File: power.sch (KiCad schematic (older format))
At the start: 32 parts, among them SW1 SW_DPST_x2, U1 SPX3819-1.8, U2 IMP811REUS-T, U3 SP6205EM5-L-3-3_TR, U4 MP1469GJ

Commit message: finished scimatic for now, and started populating PCB. *chugs rrum*
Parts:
- C1, C10, C11, C12, C13, C14, C15, C2, C3, C4, C5, C6, C7, C8, C9: footprint (none) -> Capacitor_SMD:C_0402_1005Metric
- L1, L2: footprint (none) -> Inductor_SMD:L_0402_1005Metric
- R1, R2, R3, R4, R5, R6, R7, R8, R9: footprint (none) -> Resistor_SMD:R_0402_1005Metric
- SW1, U2: footprint (none) -> Package_TO_SOT_SMD:SOT-543
- U1: footprint (none) -> Package_TO_SOT_SMD:SOT-23-5
- U4: footprint (none) -> Package_TO_SOT_SMD:SOT-223-6
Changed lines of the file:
@@
 $Descr A4 11693 8268
 encoding utf-8
-Sheet 2 4
+Sheet 2 5
 Title ""
 Date ""
@@
 F 0 "R3" V 3743 2350 50  0000 C CNN
 F 1 "100k" V 3834 2350 50  0000 C CNN
-F 2 "" V 3880 2350 50  0001 C CNN
+F 2 "Resistor_SMD:R_0402_1005Metric" V 3880 2350 50  0001 C CNN
 F 3 "~" H 3950 2350 50  0001 C CNN
 	1    3950 2350
@@
 F 0 "C10" H 5915 1946 50  0000 L CNN
 F 1 "10nF" H 5915 1855 50  0000 L CNN
-F 2 "" H 5838 1750 50  0001 C CNN
+F 2 "Capacitor_SMD:C_0402_1005Metric" H 5838 1750 50  0001 C CNN
 F 3 "~" H 5800 1900 50  0001 C CNN
 	1    5800 1900
@@
 F 0 "C9" H 5515 1946 50  0000 L CNN
 F 1 "10nF" H 5515 1855 50  0000 L CNN
-F 2 "" H 5438 1750 50  0001 C CNN
+F 2 "Capacitor_SMD:C_0402_1005Metric" H 5438 1750 50  0001 C CNN
 F 3 "~" H 5400 1900 50  0001 C CNN
 	1    5400 1900
@@
 F 0 "C2" H 2565 1946 50  0000 L CNN
 F 1 "C" H 2565 1855 50  0000 L CNN
-F 2 "" H 2488 1750 50  0001 C CNN
+F 2 "Capacitor_SMD:C_0402_1005Metric" H 2488 1750 50  0001 C CNN
 F 3 "~" H 2450 1900 50  0001 C CNN
 	1    2450 1900
@@
 F 0 "R6" V 7993 1550 50  0000 C CNN
 F 1 "33R" V 8084 1550 50  0000 C CNN
-F 2 "" V 8130 1550 50  0001 C CNN
+F 2 "Resistor_SMD:R_0402_1005Metric" V 8130 1550 50  0001 C CNN
 F 3 "~" H 8200 1550 50  0001 C CNN
 	1    8200 1550
@@
 F 0 "R9" H 8570 1796 50  0000 L CNN
 F 1 "1K" H 8570 1705 50  0000 L CNN
-F 2 "" V 8430 1750 50  0001 C CNN
+F 2 "Resistor_SMD:R_0402_1005Metric" V 8430 1750 50  0001 C CNN
 F 3 "~" H 8500 1750 50  0001 C CNN
 	1    8500 1750
@@
 F 0 "C13" H 8965 1796 50  0000 L CNN
 F 1 "10uF" H 8965 1705 50  0000 L CNN
-F 2 "" H 8888 1600 50  0001 C CNN
+F 2 "Capacitor_SMD:C_0402_1005Metric" H 8888 1600 50  0001 C CNN
 F 3 "~" H 8850 1750 50  0001 C CNN
 	1    8850 1750
@@
 F 0 "C1" H 1065 3846 50  0000 L CNN
 F 1 "100nF" H 1065 3755 50  0000 L CNN
-F 2 "" H 988 3650 50  0001 C CNN
+F 2 "Capacitor_SMD:C_0402_1005Metric" H 988 3650 50  0001 C CNN
 F 3 "~" H 950 3800 50  0001 C CNN
 	1    950  3800
@@
 F 0 "R1" V 1343 3800 50  0000 C CNN
 F 1 "100K" V 1434 3800 50  0000 C CNN
-F 2 "" V 1480 3800 50  0001 C CNN
+F 2 "Resistor_SMD:R_0402_1005Metric" V 1480 3800 50  0001 C CNN
 F 3 "~" H 1550 3800 50  0001 C CNN
 	1    1550 3800
@@
 F 0 "C3" H 3115 3996 50  0000 L CNN
 F 1 "10nF" H 3115 3905 50  0000 L CNN
-F 2 "" H 3038 3800 50  0001 C CNN
+F 2 "Capacitor_SMD:C_0402_1005Metric" H 3038 3800 50  0001 C CNN
 F 3 "~" H 3000 3950 50  0001 C CNN
 	1    3000 3950
@@
 F 0 "C5" H 3565 3996 50  0000 L CNN
 F 1 "100nF" H 3565 3905 50  0000 L CNN
-F 2 "" H 3488 3800 50  0001 C CNN
+F 2 "Capacitor_SMD:C_0402_1005Metric" H 3488 3800 50  0001 C CNN
 F 3 "~" H 3450 3950 50  0001 C CNN
 	1    3450 3950
@@
 F 0 "C6" H 4065 3996 50  0000 L CNN
 F 1 "10uF" H 4065 3905 50  0000 L CNN
-F 2 "" H 3988 3800 50  0001 C CNN
+F 2 "Capacitor_SMD:C_0402_1005Metric" H 3988 3800 50  0001 C CNN
 F 3 "~" H 3950 3950 50  0001 C CNN
 	1    3950 3950
@@
 F 0 "C7" H 5065 3946 50  0000 L CNN
 F 1 "22uF" H 5065 3855 50  0000 L CNN
-F 2 "" H 4950 3900 50  0001 C CNN
+F 2 "Capacitor_SMD:C_0402_1005Metric" H 4950 3900 50  0001 C CNN
 F 3 "~" H 4950 3900 50  0001 C CNN
 	1    4950 3900
@@
 F 0 "C8" H 5465 3946 50  0000 L CNN
 F 1 "100nF" H 5465 3855 50  0000 L CNN
-F 2 "" H 5388 3750 50  0001 C CNN
+F 2 "Capacitor_SMD:C_0402_1005Metric" H 5388 3750 50  0001 C CNN
 F 3 "~" H 5350 3900 50  0001 C CNN
 	1    5350 3900
@@
 F 0 "R4" V 5743 3850 50  0000 C CNN
 F 1 "100K" V 5834 3850 50  0000 C CNN
-F 2 "" V 5880 3850 50  0001 C CNN
+F 2 "Resistor_SMD:R_0402_1005Metric" V 5880 3850 50  0001 C CNN
 F 3 "~" H 5950 3850 50  0001 C CNN
 	1    5950 3850
@@
 F 0 "C11" V 7148 3650 50  0000 C CNN
 F 1 "1uF" V 7239 3650 50  0000 C CNN
-F 2 "" H 7438 3500 50  0001 C CNN
+F 2 "Capacitor_SMD:C_0402_1005Metric" H 7438 3500 50  0001 C CNN
 F 3 "~" H 7400 3650 50  0001 C CNN
 	1    7400 3650
@@
 F 0 "L1" V 8006 3604 50  0000 R CNN
 F 1 "3.3uH" V 7950 3750 50  0000 R CNN
-F 2 "" H 8050 3650 50  0001 C CNN
+F 2 "Inductor_SMD:L_0402_1005Metric" H 8050 3650 50  0001 C CNN
 F 3 "~" H 8050 3650 50  0001 C CNN
 	1    8050 3650
@@
 F 0 "R5" V 7443 4150 50  0000 C CNN
 F 1 "100K" V 7534 4150 50  0000 C CNN
-F 2 "" V 7580 4150 50  0001 C CNN
+F 2 "Resistor_SMD:R_0402_1005Metric" V 7580 4150 50  0001 C CNN
 F 3 "~" H 7650 4150 50  0001 C CNN
 	1    7650 4150
@@
 F 0 "R7" H 8280 3904 50  0000 R CNN
 F 1 "20K" H 8280 3995 50  0000 R CNN
-F 2 "" V 8280 3950 50  0001 C CNN
+F 2 "Resistor_SMD:R_0402_1005Metric" V 8280 3950 50  0001 C CNN
 F 3 "~" H 8350 3950 50  0001 C CNN
 	1    8350 3950
@@
 F 0 "R8" H 8280 4304 50  0000 R CNN
 F 1 "47K" H 8280 4395 50  0000 R CNN
-F 2 "" V 8280 4350 50  0001 C CNN
+F 2 "Resistor_SMD:R_0402_1005Metric" V 8280 4350 50  0001 C CNN
 F 3 "~" H 8350 4350 50  0001 C CNN
 	1    8350 4350
@@
 F 0 "C12" H 8915 3946 50  0000 L CNN
 F 1 "22uF" H 8915 3855 50  0000 L CNN
-F 2 "" H 8800 3900 50  0001 C CNN
+F 2 "Capacitor_SMD:C_0402_1005Metric" H 8800 3900 50  0001 C CNN
 F 3 "~" H 8800 3900 50  0001 C CNN
 	1    8800 3900
@@
 F 0 "C14" H 9315 3946 50  0000 L CNN
 F 1 "100nF" H 9315 3855 50  0000 L CNN
-F 2 "" H 9238 3750 50  0001 C CNN
+F 2 "Capacitor_SMD:C_0402_1005Metric" H 9238 3750 50  0001 C CNN
 F 3 "~" H 9200 3900 50  0001 C CNN
 	1    9200 3900
@@
 F 0 "L2" V 9740 3650 50  0000 C CNN
 F 1 "100r" V 9649 3650 50  0000 C CNN
-F 2 "" H 9550 3650 50  0001 C CNN
+F 2 "Inductor_SMD:L_0402_1005Metric" H 9550 3650 50  0001 C CNN
 F 3 "~" H 9550 3650 50  0001 C CNN
 	1    9550 3650
@@
 F 0 "C15" H 9965 3946 50  0000 L CNN
 F 1 "22uF" H 9965 3855 50  0000 L CNN
-F 2 "" H 9850 3900 50  0001 C CNN
+F 2 "Capacitor_SMD:C_0402_1005Metric" H 9850 3900 50  0001 C CNN
 F 3 "~" H 9850 3900 50  0001 C CNN
 	1    9850 3900
@@
 F 0 "R2" H 1820 6196 50  0000 L CNN
 F 1 "100K" H 1820 6105 50  0000 L CNN
-F 2 "" V 1680 6150 50  0001 C CNN
+F 2 "Resistor_SMD:R_0402_1005Metric" V 1680 6150 50  0001 C CNN
 F 3 "~" H 1750 6150 50  0001 C CNN
 	1    1750 6150
@@
 F 0 "C4" V 2998 5700 50  0000 C CNN
 F 1 "100nF" V 3089 5700 50  0000 C CNN
-F 2 "" H 3288 5550 50  0001 C CNN
+F 2 "Capacitor_SMD:C_0402_1005Metric" H 3288 5550 50  0001 C CNN
 F 3 "~" H 3250 5700 50  0001 C CNN
 	1    3250 5700
@@
 F 0 "U2" H 2500 5925 50  0000 C CNN
 F 1 "IMP811REUS-T" H 2500 5834 50  0000 C CNN
-F 2 "" H 2500 5700 50  0001 C CNN
+F 2 "Package_TO_SOT_SMD:SOT-543" H 2500 5700 50  0001 C CNN
 F 3 "" H 2500 5700 50  0001 C CNN
 	1    2500 5700
@@
 F 0 "U1" H 2425 3315 50  0000 C CNN
 F 1 "SPX3819-1.8" H 2425 3224 50  0000 C CNN
-F 2 "" H 2400 3300 50  0001 C CNN
+F 2 "Package_TO_SOT_SMD:SOT-23-5" H 2400 3300 50  0001 C CNN
 F 3 "" H 2400 3300 50  0001 C CNN
 	1    2400 3300
@@
 F 0 "U4" H 6650 3375 50  0000 C CNN
 F 1 "MP1469GJ" H 6650 3284 50  0000 C CNN
-F 2 "" H 6650 3400 50  0001 C CNN
+F 2 "Package_TO_SOT_SMD:SOT-223-6" H 6650 3400 50  0001 C CNN
 F 3 "" H 6650 3400 50  0001 C CNN
 	1    6650 3400
@@
 F 0 "SW1" H 4800 6335 50  0000 C CNN
 F 1 "SW_DPST_x2" H 4800 6244 50  0000 C CNN
-F 2 "" H 4800 6100 50  0001 C CNN
+F 2 "Package_TO_SOT_SMD:SOT-543" H 4800 6100 50  0001 C CNN
 F 3 "~" H 4800 6100 50  0001 C CNN
 	1    4800 6100

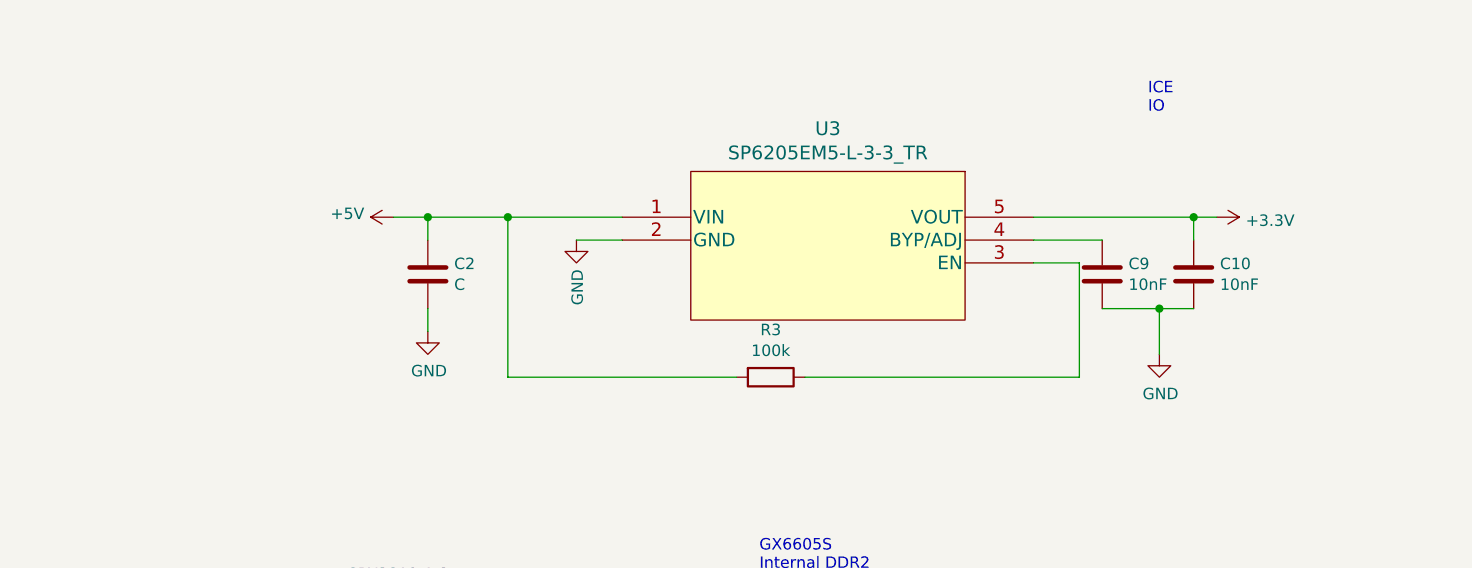
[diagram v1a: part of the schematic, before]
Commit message: started layout of the PCB, allso moved onto craken rum, from captin morgan. please for the love of god check the footprints are right. @MAX
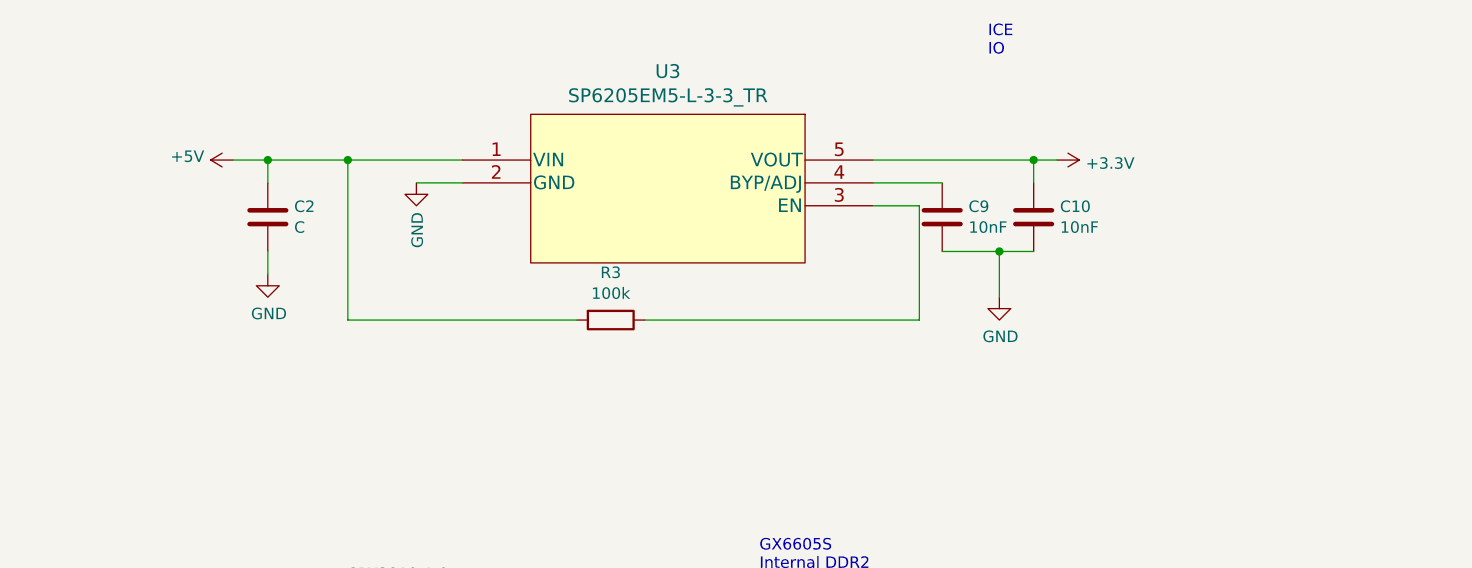
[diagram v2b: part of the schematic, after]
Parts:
- SW1: footprint Package_TO_SOT_SMD:SOT-543 -> Jumper:SolderJumper-2_P1.3mm_Open_Pad1.0x1.5mm
- U3: footprint SOT-23-5_VAR-AA -> Package_TO_SOT_SMD:SOT-23-5
- U4: footprint Package_TO_SOT_SMD:SOT-223-6 -> Package_TO_SOT_SMD:SOT-23-6
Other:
- moved on the sheet: C10, C2, C9, R3, U3
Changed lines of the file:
@@
 $EndDescr
 Wire Wire Line
-	3300 1650 2800 1650
-Wire Wire Line
-	2800 1650 2800 2350
-Wire Wire Line
-	5300 2350 5300 1850
-Wire Wire Line
-	5300 1850 5100 1850
-Connection ~ 2800 1650
-Wire Wire Line
-	2800 1650 2450 1650
+	2600 1400 2100 1400
+Wire Wire Line
+	2100 1400 2100 2100
+Wire Wire Line
+	4600 2100 4600 1600
+Wire Wire Line
+	4600 1600 4400 1600
+Connection ~ 2100 1400
+Wire Wire Line
+	2100 1400 1750 1400
 $Comp
 L power:GND #PWR0101
 U 1 1 5F46AF52
-P 3100 1750
-F 0 "#PWR0101" H 3100 1500 50  0001 C CNN
-F 1 "GND" V 3105 1622 50  0000 R CNN
-F 2 "" H 3100 1750 50  0001 C CNN
-F 3 "" H 3100 1750 50  0001 C CNN
-	1    3100 1750
-	1    0    0    -1
-$EndComp
-Wire Wire Line
-	3100 1750 3300 1750
+P 2400 1500
+F 0 "#PWR0101" H 2400 1250 50  0001 C CNN
+F 1 "GND" V 2405 1372 50  0000 R CNN
+F 2 "" H 2400 1500 50  0001 C CNN
+F 3 "" H 2400 1500 50  0001 C CNN
+	1    2400 1500
+	1    0    0    -1
+$EndComp
+Wire Wire Line
+	2400 1500 2600 1500
 $Comp
 L power:+5V #PWR0102
 U 1 1 5F46BAA8
-P 2300 1650
-F 0 "#PWR0102" H 2300 1500 50  0001 C CNN
-F 1 "+5V" V 2315 1778 50  0000 L CNN
-F 2 "" H 2300 1650 50  0001 C CNN
-F 3 "" H 2300 1650 50  0001 C CNN
-	1    2300 1650
+P 1600 1400
+F 0 "#PWR0102" H 1600 1250 50  0001 C CNN
+F 1 "+5V" V 1615 1528 50  0000 L CNN
+F 2 "" H 1600 1400 50  0001 C CNN
+F 3 "" H 1600 1400 50  0001 C CNN
+	1    1600 1400
 	0    -1   -1   0
 $EndComp
@@
 L power:+3.3V #PWR0103
 U 1 1 5F46C36C
-P 5900 1650
-F 0 "#PWR0103" H 5900 1500 50  0001 C CNN
-F 1 "+3.3V" V 5915 1778 50  0000 L CNN
-F 2 "" H 5900 1650 50  0001 C CNN
-F 3 "" H 5900 1650 50  0001 C CNN
-	1    5900 1650
+P 5200 1400
+F 0 "#PWR0103" H 5200 1250 50  0001 C CNN
+F 1 "+3.3V" V 5215 1528 50  0000 L CNN
+F 2 "" H 5200 1400 50  0001 C CNN
+F 3 "" H 5200 1400 50  0001 C CNN
+	1    5200 1400
 	0    1    1    0
 $EndComp
 Wire Wire Line
-	5100 1750 5400 1750
+	4400 1500 4700 1500
 $Comp
 L power:GND #PWR0104
 U 1 1 5F46E6EF
-P 5650 2250
-F 0 "#PWR0104" H 5650 2000 50  0001 C CNN
-F 1 "GND" H 5655 2077 50  0000 C CNN
-F 2 "" H 5650 2250 50  0001 C CNN
-F 3 "" H 5650 2250 50  0001 C CNN
-	1    5650 2250
-	1    0    0    -1
-$EndComp
-Wire Wire Line
-	5650 2050 5650 2250
-Wire Wire Line
-	5800 2050 5650 2050
-Wire Wire Line
-	5800 1750 5800 1650
-Wire Wire Line
-	5800 1650 5900 1650
-Wire Wire Line
-	5800 1650 5100 1650
-Connection ~ 5800 1650
+P 4950 2000
+F 0 "#PWR0104" H 4950 1750 50  0001 C CNN
+F 1 "GND" H 4955 1827 50  0000 C CNN
+F 2 "" H 4950 2000 50  0001 C CNN
+F 3 "" H 4950 2000 50  0001 C CNN
+	1    4950 2000
+	1    0    0    -1
+$EndComp
+Wire Wire Line
+	4950 1800 4950 2000
+Wire Wire Line
+	5100 1800 4950 1800
+Wire Wire Line
+	5100 1500 5100 1400
+Wire Wire Line
+	5100 1400 5200 1400
+Wire Wire Line
+	5100 1400 4400 1400
+Connection ~ 5100 1400
 $Comp
 L Device:R R3
 U 1 1 5F46F847
-P 3950 2350
-F 0 "R3" V 3743 2350 50  0000 C CNN
-F 1 "100k" V 3834 2350 50  0000 C CNN
-F 2 "Resistor_SMD:R_0402_1005Metric" V 3880 2350 50  0001 C CNN
-F 3 "~" H 3950 2350 50  0001 C CNN
-	1    3950 2350
+P 3250 2100
+F 0 "R3" V 3043 2100 50  0000 C CNN
+F 1 "100k" V 3134 2100 50  0000 C CNN
+F 2 "Resistor_SMD:R_0402_1005Metric" V 3180 2100 50  0001 C CNN
+F 3 "~" H 3250 2100 50  0001 C CNN
+	1    3250 2100
 	0    1    1    0
 $EndComp
 Wire Wire Line
-	5300 2350 4100 2350
-Wire Wire Line
-	2800 2350 3800 2350
+	4600 2100 3400 2100
+Wire Wire Line
+	2100 2100 3100 2100
 $Comp
 L Device:C C10
 U 1 1 5F46E13B
-P 5800 1900
-F 0 "C10" H 5915 1946 50  0000 L CNN
-F 1 "10nF" H 5915 1855 50  0000 L CNN
-F 2 "Capacitor_SMD:C_0402_1005Metric" H 5838 1750 50  0001 C CNN
-F 3 "~" H 5800 1900 50  0001 C CNN
-	1    5800 1900
-	1    0    0    -1
-$EndComp
-Connection ~ 5650 2050
+P 5100 1650
+F 0 "C10" H 5215 1696 50  0000 L CNN
+F 1 "10nF" H 5215 1605 50  0000 L CNN
+F 2 "Capacitor_SMD:C_0402_1005Metric" H 5138 1500 50  0001 C CNN
+F 3 "~" H 5100 1650 50  0001 C CNN
+	1    5100 1650
+	1    0    0    -1
+$EndComp
+Connection ~ 4950 1800
 $Comp
 L Device:C C9
 U 1 1 5F46CE59
-P 5400 1900
-F 0 "C9" H 5515 1946 50  0000 L CNN
-F 1 "10nF" H 5515 1855 50  0000 L CNN
-F 2 "Capacitor_SMD:C_0402_1005Metric" H 5438 1750 50  0001 C CNN
-F 3 "~" H 5400 1900 50  0001 C CNN
-	1    5400 1900
-	1    0    0    -1
-$EndComp
-Wire Wire Line
-	5400 2050 5650 2050
+P 4700 1650
+F 0 "C9" H 4815 1696 50  0000 L CNN
+F 1 "10nF" H 4815 1605 50  0000 L CNN
+F 2 "Capacitor_SMD:C_0402_1005Metric" H 4738 1500 50  0001 C CNN
+F 3 "~" H 4700 1650 50  0001 C CNN
+	1    4700 1650
+	1    0    0    -1
+$EndComp
+Wire Wire Line
+	4700 1800 4950 1800
 $Comp
 L power:GND #PWR0105
 U 1 1 5F4AC863
-P 2450 2150
-F 0 "#PWR0105" H 2450 1900 50  0001 C CNN
-F 1 "GND" H 2455 1977 50  0000 C CNN
-F 2 "" H 2450 2150 50  0001 C CNN
-F 3 "" H 2450 2150 50  0001 C CNN
-	1    2450 2150
+P 1750 1900
+F 0 "#PWR0105" H 1750 1650 50  0001 C CNN
+F 1 "GND" H 1755 1727 50  0000 C CNN
+F 2 "" H 1750 1900 50  0001 C CNN
+F 3 "" H 1750 1900 50  0001 C CNN
+	1    1750 1900
 	1    0    0    -1
 $EndComp
@@
 L Device:C C2
 U 1 1 5F4ACF4B
-P 2450 1900
-F 0 "C2" H 2565 1946 50  0000 L CNN
-F 1 "C" H 2565 1855 50  0000 L CNN
-F 2 "Capacitor_SMD:C_0402_1005Metric" H 2488 1750 50  0001 C CNN
-F 3 "~" H 2450 1900 50  0001 C CNN
-	1    2450 1900
+P 1750 1650
+F 0 "C2" H 1865 1696 50  0000 L CNN
+F 1 "C" H 1865 1605 50  0000 L CNN
+F 2 "Capacitor_SMD:C_0402_1005Metric" H 1788 1500 50  0001 C CNN
+F 3 "~" H 1750 1650 50  0001 C CNN
+	1    1750 1650
 	1    0    0    -1
 $EndComp
@@
 L Csky:SP6205EM5-L-3-3_TR U3
 U 1 1 5F4A6E5D
-P 3300 1650
-F 0 "U3" H 4200 2037 60  0000 C CNN
-F 1 "SP6205EM5-L-3-3_TR" H 4200 1931 60  0000 C CNN
-F 2 "SOT-23-5_VAR-AA" H 4200 1890 60  0001 C CNN
-F 3 "" H 3300 1650 60  0000 C CNN
-	1    3300 1650
-	1    0    0    -1
-$EndComp
-Wire Wire Line
-	2450 2150 2450 2050
-Wire Wire Line
-	2450 1750 2450 1650
-Connection ~ 2450 1650
-Wire Wire Line
-	2450 1650 2300 1650
+P 2600 1400
+F 0 "U3" H 3500 1787 60  0000 C CNN
+F 1 "SP6205EM5-L-3-3_TR" H 3500 1681 60  0000 C CNN
+F 2 "Package_TO_SOT_SMD:SOT-23-5" H 3500 1640 60  0001 C CNN
+F 3 "" H 2600 1400 60  0000 C CNN
+	1    2600 1400
+	1    0    0    -1
+$EndComp
+Wire Wire Line
+	1750 1900 1750 1800
+Wire Wire Line
+	1750 1500 1750 1400
+Connection ~ 1750 1400
+Wire Wire Line
+	1750 1400 1600 1400
 Text Notes 9050 1300 0    50   ~ 0
 HDMI\n
-Text Notes 5600 1200 0    50   ~ 0
+Text Notes 4900 950  0    50   ~ 0
 ICE\nIO
 $Comp
@@
 F 0 "U4" H 6650 3375 50  0000 C CNN
 F 1 "MP1469GJ" H 6650 3284 50  0000 C CNN
-F 2 "Package_TO_SOT_SMD:SOT-223-6" H 6650 3400 50  0001 C CNN
+F 2 "Package_TO_SOT_SMD:SOT-23-6" H 6650 3400 50  0001 C CNN
 F 3 "" H 6650 3400 50  0001 C CNN
 	1    6650 3400
@@
 F 0 "SW1" H 4800 6335 50  0000 C CNN
 F 1 "SW_DPST_x2" H 4800 6244 50  0000 C CNN
-F 2 "Package_TO_SOT_SMD:SOT-543" H 4800 6100 50  0001 C CNN
+F 2 "Jumper:SolderJumper-2_P1.3mm_Open_Pad1.0x1.5mm" H 4800 6100 50  0001 C CNN
 F 3 "~" H 4800 6100 50  0001 C CNN
 	1    4800 6100
